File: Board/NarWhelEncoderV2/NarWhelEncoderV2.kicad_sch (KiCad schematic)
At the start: 35 parts, among them IC1 AS5047U-HTSM, IC2 SN65LVDS049PWR, IC3 LM1117-3.3, J1 HX_3p, J2 DS1128-09-S8B8X, J3 DS1128-09-S8B8X, Q1 2N7002, Q2 2N7002

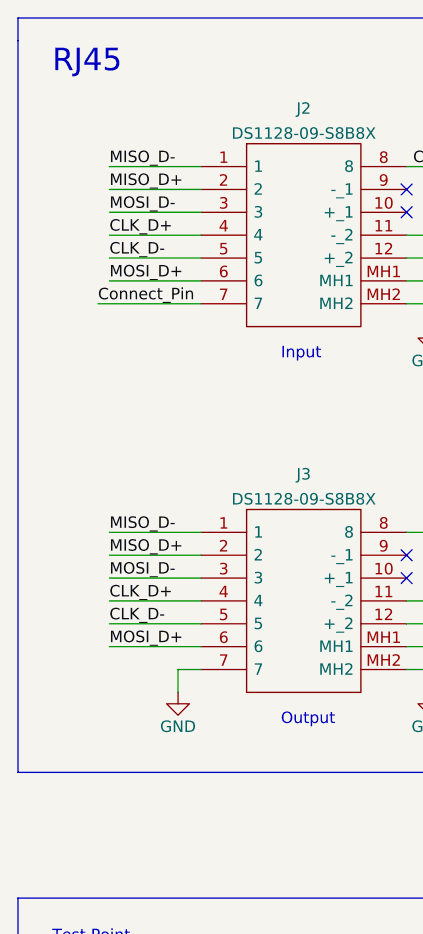
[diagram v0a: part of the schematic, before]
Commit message: Update Board
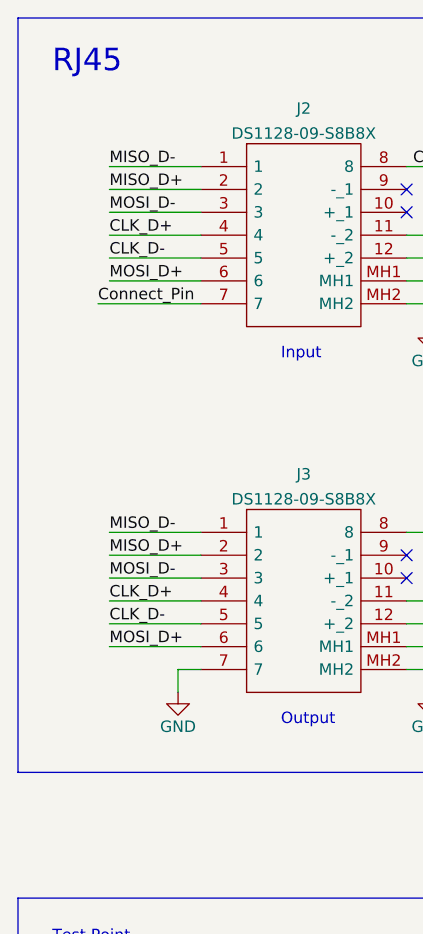
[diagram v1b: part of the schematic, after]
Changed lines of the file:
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@@
     (stroke (width 0) (type default) (color 0 0 0 0))
   )
-  (polyline (pts (xy 24.13 25.4) (xy 24.13 106.68))
+  (polyline (pts (xy 24.13 22.86) (xy 24.13 106.68))
     (stroke (width 0) (type default) (color 0 0 0 0))
   )
@@
     (stroke (width 0) (type default) (color 0 0 0 0))
   )
-  (polyline (pts (xy 24.13 22.86) (xy 24.13 25.4))
+  (polyline (pts (xy 24.13 22.86) (xy 24.13 22.86))
     (stroke (width 0) (type default) (color 0 0 0 0))
   )
